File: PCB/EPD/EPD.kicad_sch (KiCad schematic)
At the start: 68 parts, among them J1 Conn_01x26, J2 Shelly, J3 USB-PROG, J4 BTN1, J6 BTN2, J7 USB-C-Socket-V, J8 PWR, P1 +, P10 2, P11 1, P12 1, P2 -, P3 2, P4 2, P5 1, P6 1, P7 +, P8 -, P9 2, Q1 DMG1012T, U2 ESP32-S3-MINI-1, U3 MD8942

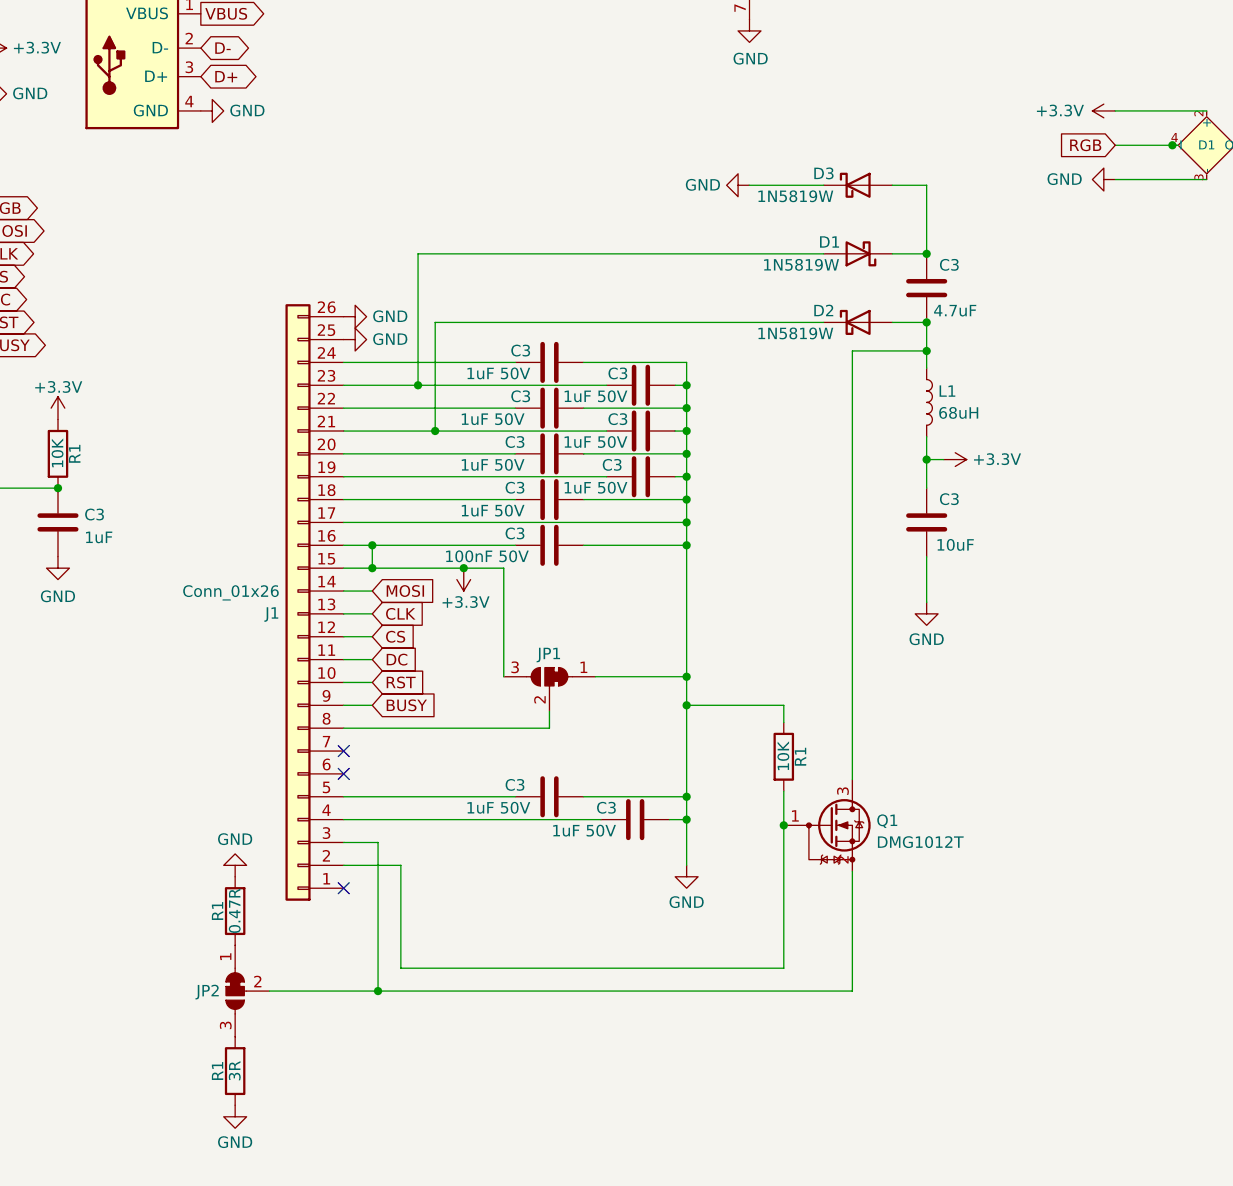
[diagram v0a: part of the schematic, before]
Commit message: Updated
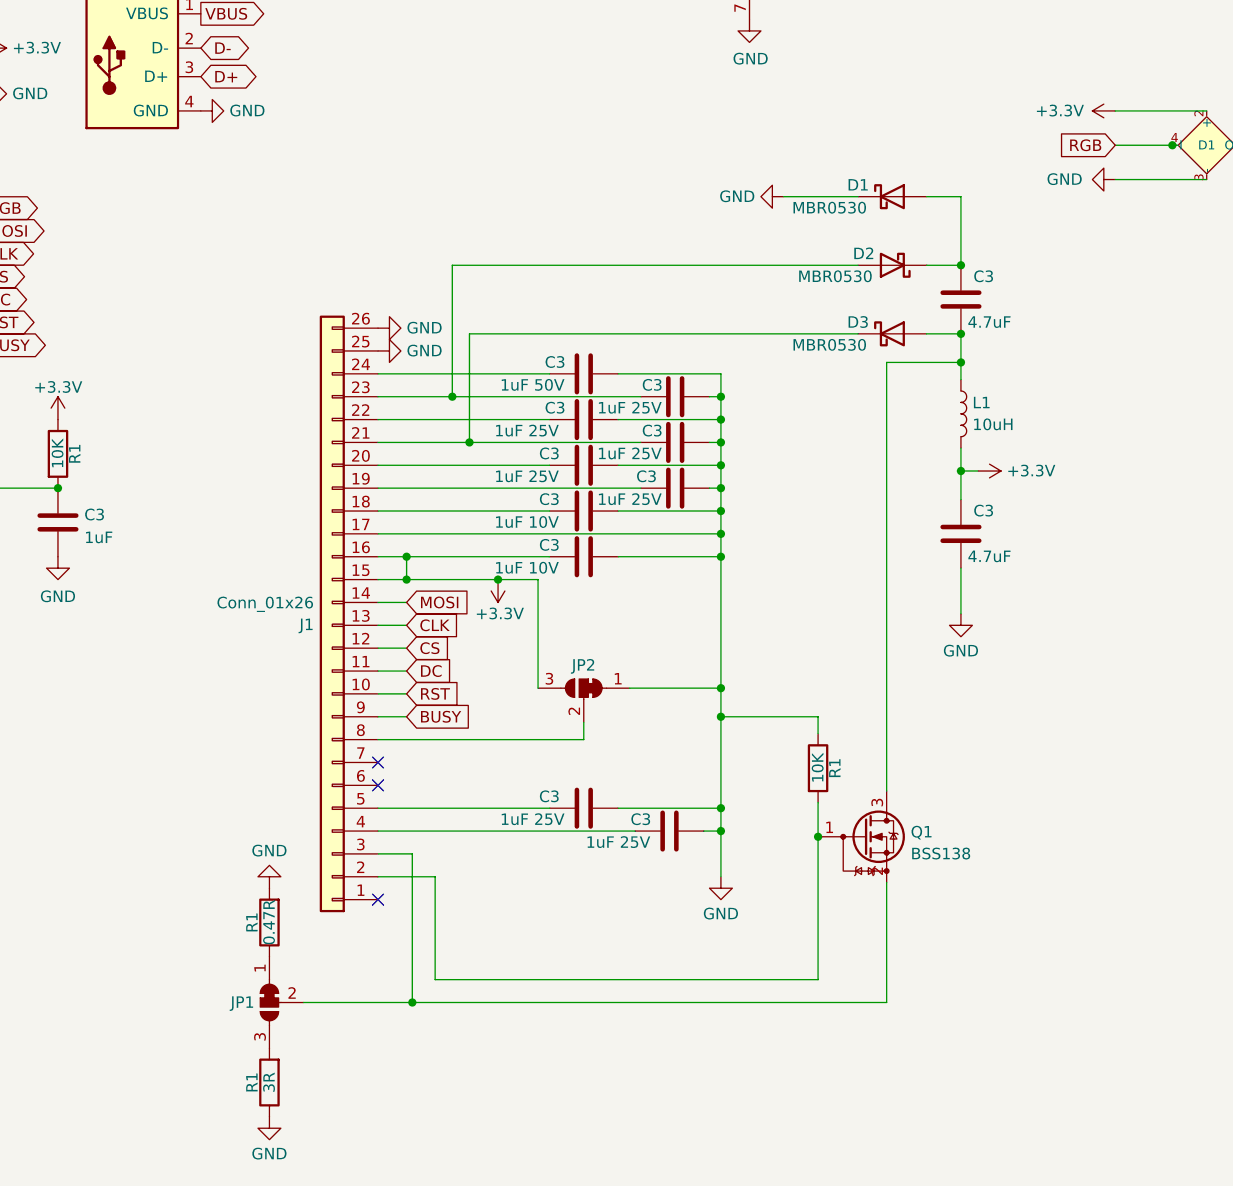
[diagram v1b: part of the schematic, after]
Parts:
- removed C3 (x9): 1uF 50V, RevK:C_0402, symbol Device:C
- removed C3: 100nF 50V, RevK:C_0402, symbol Device:C
- removed C3: 4.7uF, RevK:C_0402, symbol Device:C
- removed C3: 10uF, RevK:C_0402, symbol Device:C
- removed R1: 10K, RevK:R_0402, symbol Device:R
- removed R1: 0.47R, RevK:R_0402, symbol Device:R
- removed R1: 3R, RevK:R_0402, symbol Device:R
- added C3 (x7): 1uF 25V, RevK:C_0402, symbol Device:C
- added C3 (x2): 1uF 10V, RevK:C_0402, symbol Device:C
- added C3: 1uF 50V, RevK:C_0402, symbol Device:C
- added C3 (x2): 4.7uF, RevK:C_0402, symbol Device:C
- added R1: 0.47R, RevK:R_0402, symbol Device:R
- added R1: 10K, RevK:R_0402, symbol Device:R
- added R1: 3R, RevK:R_0402, symbol Device:R
- D1, D2, D3: value 1N5819W -> MBR0530; LCSC Part # C2905650 -> C5204746
- L1: value 68uH -> 10uH; footprint RevK:L_0805 -> RevK:L_4x4; LCSC Part # C275376 -> C38117
- Q1: value DMG1012T -> BSS138; footprint RevK:SOT-323_SC-70-3 -> RevK:SOT-23; LCSC Part # C469327 -> C5279927
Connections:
- net +3.3V: now also JP2.3 (B), C3.1, C3.2; no longer JP1.3 (B)
- net GND: now also D1.1 (K), JP2.1 (A), C3.1, C3.2, C3.2, C3.2, C3.2, C3.2, C3.2, C3.2, C3.2, C3.2, C3.2, R1.1, R1.1, R1.2; no longer D3.1 (K), JP1.1 (A)
- net at J1.2 (Pin_2), Q1.1 (G): now also R1.2
- net at J1.3 (Pin_3), Q1.2 (S): now also JP1.2 (C); no longer JP2.2 (C)
- net at L1.1, Q1.3 (D): now also D3.2 (A), C3.1; no longer D2.2 (A)
- net at D1.2 (A): now also D2.1 (K), C3.2; no longer J1.23 (Pin_23)
- net at J1.5 (Pin_5): now also C3.1
- net at J1.21 (Pin_21): now also D3.1 (K), C3.1; no longer D2.1 (K)
- net at J1.22 (Pin_22): now also C3.1
- net at J1.18 (Pin_18): now also C3.1
- net at J1.19 (Pin_19): now also C3.1
- net at J1.20 (Pin_20): now also C3.1
- net at J1.24 (Pin_24): now also C3.1
- net at J1.4 (Pin_4): now also C3.1
- net at J1.8 (Pin_8): now also JP2.2 (C); no longer JP1.2 (C)
- new net: JP1.1 (A), R1.1
- new net: C3.1, D2.2 (A), J1.23 (Pin_23)
- new net: JP1.3 (B), R1.2
